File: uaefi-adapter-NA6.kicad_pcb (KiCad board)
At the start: 2 copper layers, 154 x 159 mm, 64 parts, among them J11 Conn_01x01, J13 Conn_01x01, J14 Conn_01x01, J15 Conn_01x01, J16 Conn_01x01, J17 Conn_01x01, P10 Pad, P15 Pad, P16 Pad, P17 Pad, P19 Pad, P2 178780-1, P21 Pad, P3 Pad, P46 Pad, P7 Pad, P8 Pad, P9 Pad

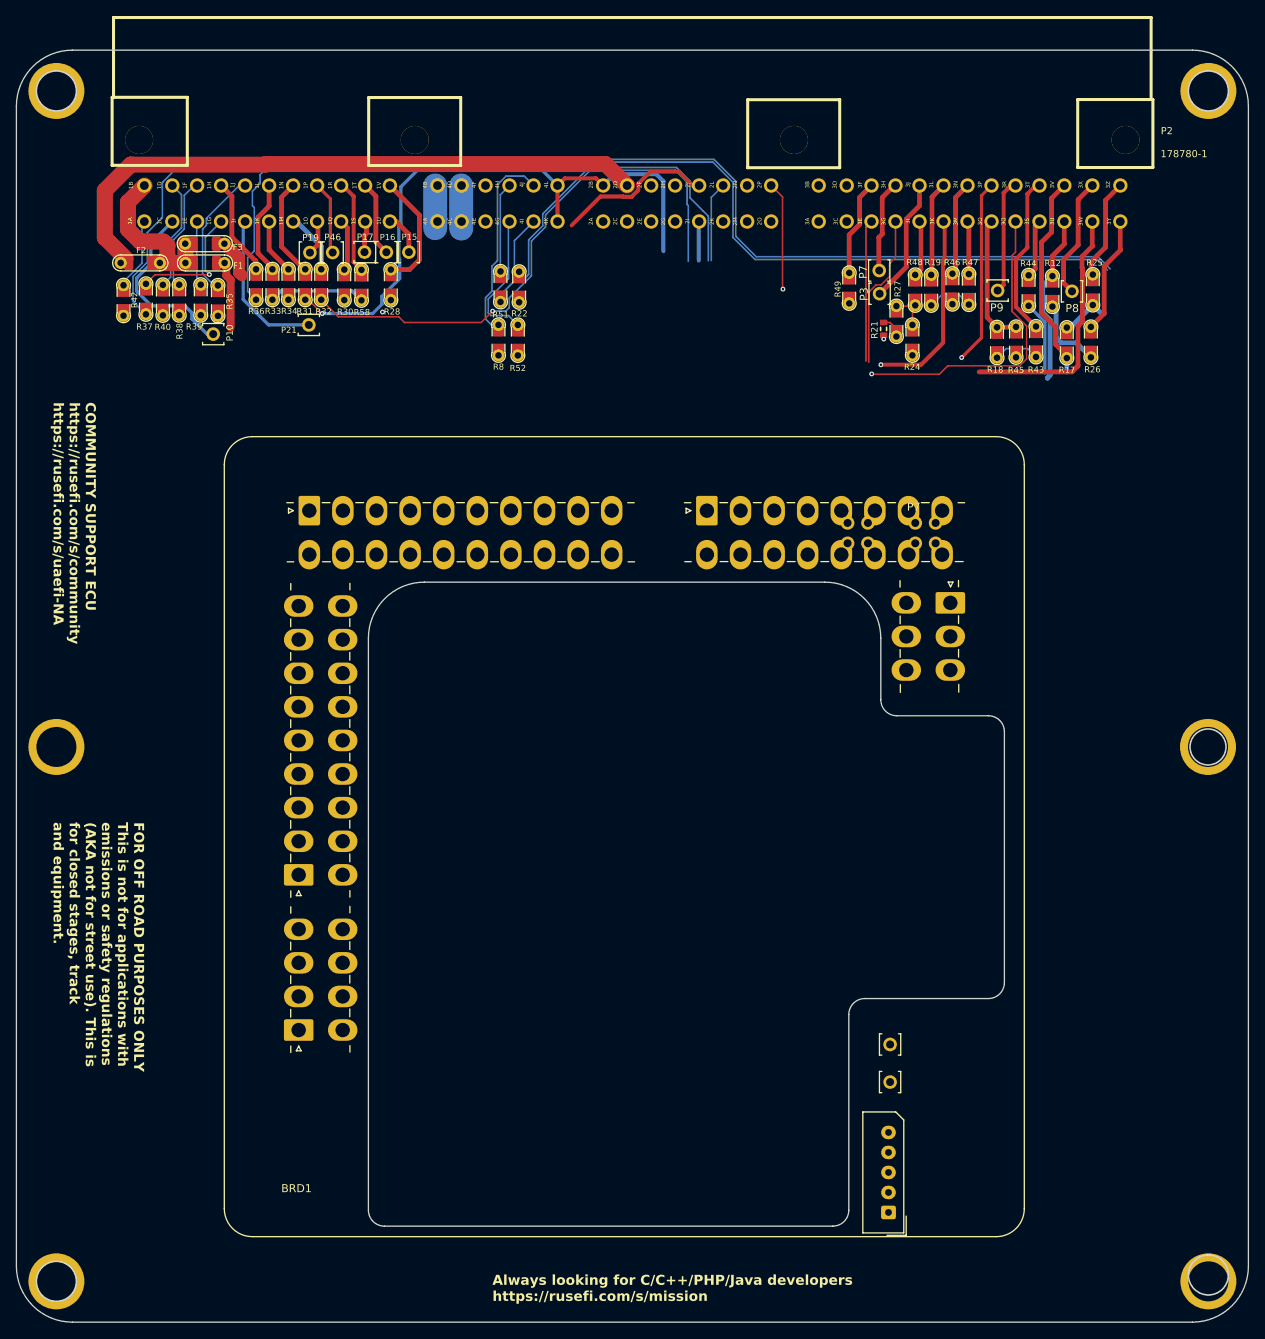
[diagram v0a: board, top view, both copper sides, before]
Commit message: upd
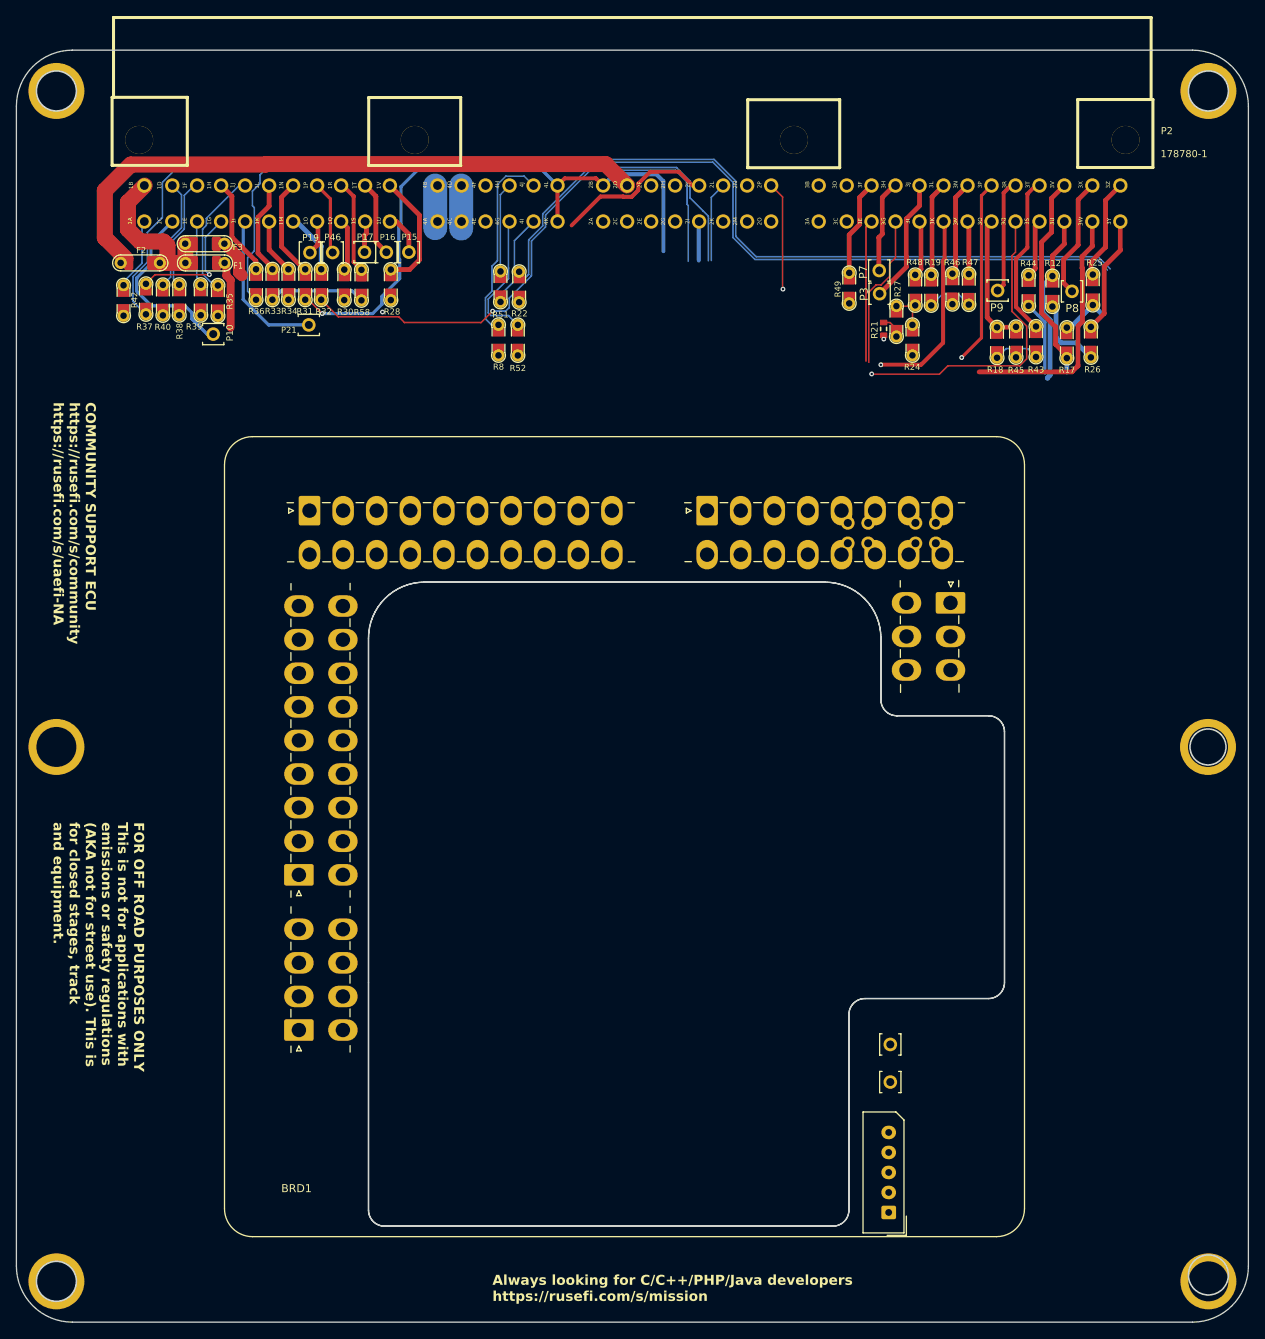
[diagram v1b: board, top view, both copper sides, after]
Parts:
- removed the P7 at (135.4, 82.6)
- removed the P7 at (132.9, 82.6)
- removed the P7 at (126.9, 82.6)
- removed the P7 at (126.9, 80.1)
- removed the P7 at (124.4, 80.1)
- removed the P7 at (132.9, 80.1)
- removed the P7 at (124.4, 82.6)
- removed the P7 at (135.4, 80.1)
